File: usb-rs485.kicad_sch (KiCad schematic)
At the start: 8 parts

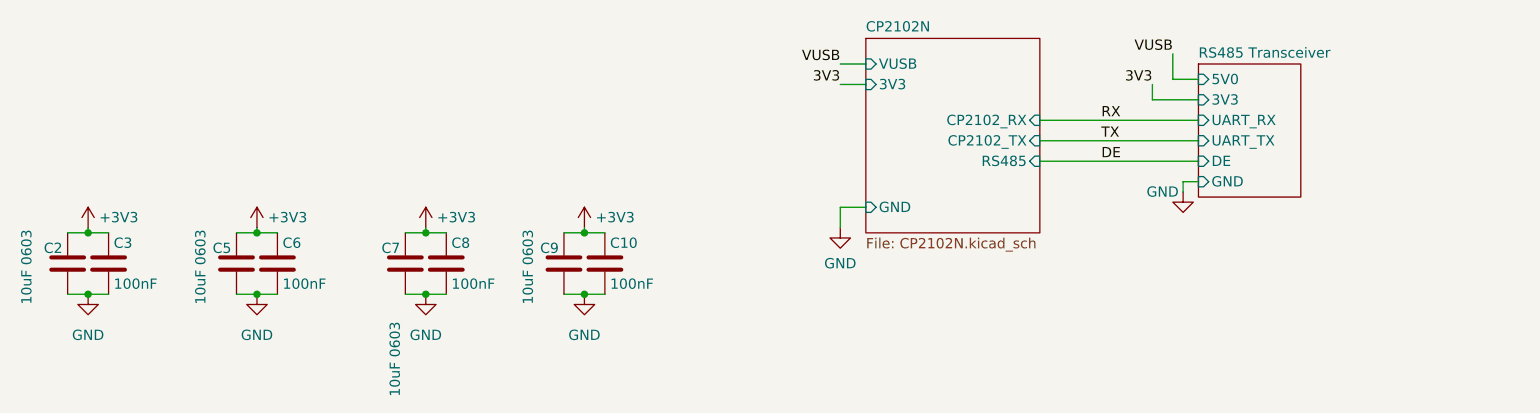
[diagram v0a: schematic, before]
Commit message: routing
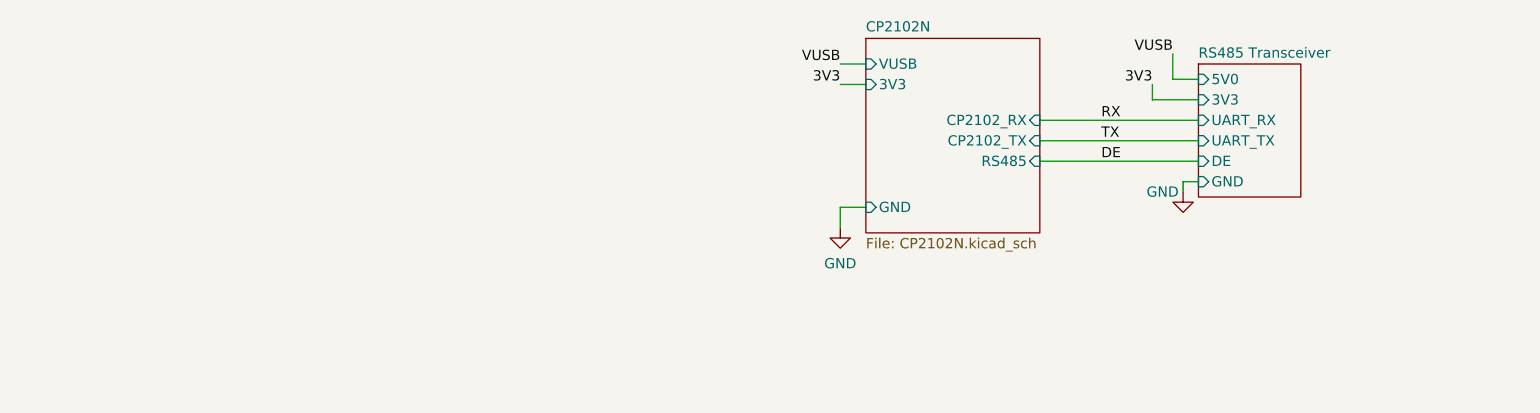
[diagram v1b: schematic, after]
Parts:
- removed C10, C3, C6, C8: 100nF, robot-cortex:C_0402_1005Metric, symbol usb-rs485:Capacitor
- removed C2, C5, C7, C9: 10uF 0603, robot-cortex:C_0603_1608Metric, symbol usb-rs485:Capacitor

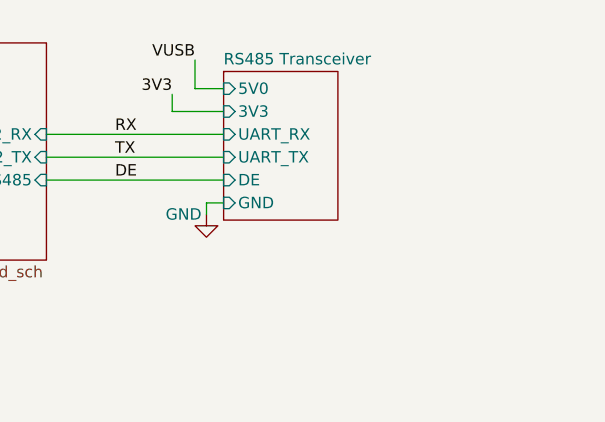
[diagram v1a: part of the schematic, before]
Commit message: routed, thru holes. ready to order i think
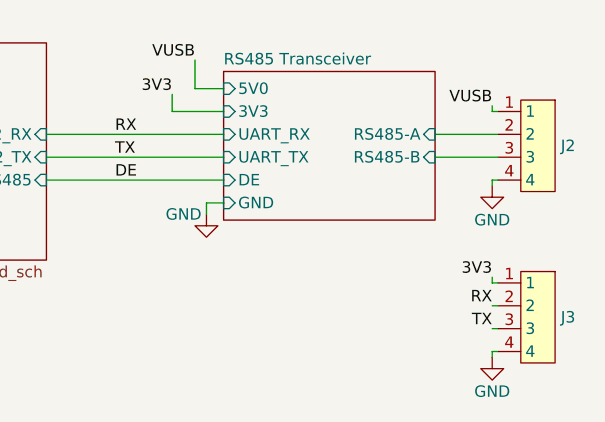
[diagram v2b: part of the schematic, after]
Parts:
- added J2, J3: ~, robot-cortex:ThruHoleBreadboardX4, symbol usb-rs485:ThruHoleX4
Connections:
- net 3V3: now also J3.1
- net GND: now also J2.4, J3.4
- net RX: now also J3.2
- net TX: now also J3.3
- net VUSB: now also J2.1
- new net RS485 Transceiver/RS485-A: J2.2
- new net RS485 Transceiver/RS485-B: J2.3
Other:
- sheet RS485 Transceiver ports: added RS485-A, RS485-B; removed none
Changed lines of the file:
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@@
 (kicad_sch (version 20230121) (generator eeschema)
   (paper "A3")
+  (wire (pts (xy 328.93 173.99) (xy 328.93 174.625))
+    (stroke (width 0) (type default))
+  )
+  (wire (pts (xy 328.93 154.94) (xy 328.93 155.575))
+    (stroke (width 0) (type default))
+  )
   (wire (pts (xy 295.91 144.78) (xy 299.085 144.78))
     (stroke (width 0) (type default))
   )
+  (wire (pts (xy 328.93 166.37) (xy 329.565 166.37))
+    (stroke (width 0) (type default))
+  )
+  (wire (pts (xy 328.93 173.99) (xy 329.565 173.99))
+    (stroke (width 0) (type default))
+  )
+  (wire (pts (xy 328.93 165.735) (xy 328.93 166.37))
+    (stroke (width 0) (type default))
+  )
   (wire (pts (xy 279.4 152.4) (xy 299.085 152.4))
     (stroke (width 0) (type default))
@@
     (stroke (width 0) (type default))
   )
+  (wire (pts (xy 322.58 149.86) (xy 329.565 149.86))
+    (stroke (width 0) (type default))
+  )
+  (wire (pts (xy 328.93 147.32) (xy 329.565 147.32))
+    (stroke (width 0) (type default))
+  )
   (wire (pts (xy 295.91 144.78) (xy 295.91 141.605))
     (stroke (width 0) (type default))
@@
     (stroke (width 0) (type default))
   )
+  (wire (pts (xy 322.58 152.4) (xy 329.565 152.4))
+    (stroke (width 0) (type default))
+  )
   (wire (pts (xy 279.4 149.86) (xy 299.085 149.86))
     (stroke (width 0) (type default))
   )
+  (wire (pts (xy 328.93 168.91) (xy 329.565 168.91))
+    (stroke (width 0) (type default))
+  )
+  (wire (pts (xy 328.93 171.45) (xy 329.565 171.45))
+    (stroke (width 0) (type default))
+  )
   (wire (pts (xy 297.18 157.48) (xy 297.18 158.75))
     (stroke (width 0) (type default))
@@
     (stroke (width 0) (type default))
   )
+  (wire (pts (xy 328.93 146.685) (xy 328.93 147.32))
+    (stroke (width 0) (type default))
+  )
+  (wire (pts (xy 328.93 154.94) (xy 329.565 154.94))
+    (stroke (width 0) (type default))
+  )
   (label "VUSB" (at 254.635 142.875 180) (fields_autoplaced)
+    (effects (font (size 1.27 1.27)) (justify right bottom))
+  )
+  (label "TX" (at 328.93 171.45 180) (fields_autoplaced)
     (effects (font (size 1.27 1.27)) (justify right bottom))
   )
@@
     (effects (font (size 1.27 1.27)) (justify right bottom))
   )
+  (label "RX" (at 328.93 168.91 180) (fields_autoplaced)
+    (effects (font (size 1.27 1.27)) (justify right bottom))
+  )
   (label "3V3" (at 293.37 145.415 180) (fields_autoplaced)
     (effects (font (size 1.27 1.27)) (justify right bottom))
@@
   (label "RX" (at 287.02 149.86 0) (fields_autoplaced)
     (effects (font (size 1.27 1.27)) (justify left bottom))
+  )
+  (label "VUSB" (at 328.93 146.685 180) (fields_autoplaced)
+    (effects (font (size 1.27 1.27)) (justify right bottom))
+  )
+  (label "3V3" (at 328.93 165.735 180) (fields_autoplaced)
+    (effects (font (size 1.27 1.27)) (justify right bottom))
   )
   (symbol (lib_id "power:GND") (at 297.18 158.75 0) (unit 1)
@@
     )
   )
-  (sheet (at 299.085 142.875) (size 12.7 16.51)
+  (symbol (lib_id "power:GND") (at 328.93 155.575 0) (unit 1)
+    (in_bom yes) (on_board yes) (dnp no)
+    (property "Reference" "#PWR011" (at 328.93 161.925 0)
+      (effects (font (size 1.27 1.27)) hide)
+    )
+    (property "Value" "GND" (at 328.93 159.385 0)
+      (effects (font (size 1.27 1.27)))
+    )
+    (property "Footprint" "" (at 328.93 155.575 0)
+      (effects (font (size 1.27 1.27)) hide)
+    )
+    (property "Datasheet" "" (at 328.93 155.575 0)
+      (effects (font (size 1.27 1.27)) hide)
+    )
+    (pin "1")
+    (instances
+      (project "usb-rs485"
+        (path "/19e4cb9f-d0a4-4ce0-8aa4-5fe95563dc37"
+          (reference "#PWR011") (unit 1)
+        )
+      )
+    )
+  )
+  (symbol (lib_id "usb-rs485:ThruHoleX4") (at 332.105 170.18 0) (mirror y) (unit 1)
+    (in_bom no) (on_board yes) (dnp no) (fields_autoplaced)
+    (property "Reference" "J3" (at 336.55 170.18 0)
+      (effects (font (size 1.27 1.27)) (justify right))
+    )
+    (property "Value" "~" (at 330.835 168.91 0)
+      (effects (font (size 1.27 1.27)))
+    )
+    (property "Footprint" "robot-cortex:ThruHoleBreadboardX4" (at 330.835 168.91 0)
+      (effects (font (size 1.27 1.27)) hide)
+    )
+    (property "Datasheet" "" (at 330.835 168.91 0)
+      (effects (font (size 1.27 1.27)) hide)
+    )
+    (pin "3")
+    (pin "4")
+    (pin "2")
+    (pin "1")
+    (instances
+      (project "usb-rs485"
+        (path "/19e4cb9f-d0a4-4ce0-8aa4-5fe95563dc37"
+          (reference "J3") (unit 1)
+        )
+      )
+    )
+  )
+  (symbol (lib_id "usb-rs485:ThruHoleX4") (at 332.105 151.13 0) (mirror y) (unit 1)
+    (in_bom no) (on_board yes) (dnp no) (fields_autoplaced)
+    (property "Reference" "J2" (at 336.55 151.13 0)
+      (effects (font (size 1.27 1.27)) (justify right))
+    )
+    (property "Value" "~" (at 330.835 149.86 0)
+      (effects (font (size 1.27 1.27)))
+    )
+    (property "Footprint" "robot-cortex:ThruHoleBreadboardX4" (at 330.835 149.86 0)
+      (effects (font (size 1.27 1.27)) hide)
+    )
+    (property "Datasheet" "" (at 330.835 149.86 0)
+      (effects (font (size 1.27 1.27)) hide)
+    )
+    (pin "3")
+    (pin "4")
+    (pin "2")
+    (pin "1")
+    (instances
+      (project "usb-rs485"
+        (path "/19e4cb9f-d0a4-4ce0-8aa4-5fe95563dc37"
+          (reference "J2") (unit 1)
+        )
+      )
+    )
+  )
+  (symbol (lib_id "power:GND") (at 328.93 174.625 0) (unit 1)
+    (in_bom yes) (on_board yes) (dnp no)
+    (property "Reference" "#PWR012" (at 328.93 180.975 0)
+      (effects (font (size 1.27 1.27)) hide)
+    )
+    (property "Value" "GND" (at 328.93 178.435 0)
+      (effects (font (size 1.27 1.27)))
+    )
+    (property "Footprint" "" (at 328.93 174.625 0)
+      (effects (font (size 1.27 1.27)) hide)
+    )
+    (property "Datasheet" "" (at 328.93 174.625 0)
+      (effects (font (size 1.27 1.27)) hide)
+    )
+    (pin "1")
+    (instances
+      (project "usb-rs485"
+        (path "/19e4cb9f-d0a4-4ce0-8aa4-5fe95563dc37"
+          (reference "#PWR012") (unit 1)
+        )
+      )
+    )
+  )
+  (sheet (at 299.085 142.875) (size 23.495 16.51)
     (stroke (width 0.1524) (type solid))
     (fill (color 0 0 0 0.0000))
@@
       (effects (font (size 1.27 1.27)) (justify left))
     )
-    (instances
+    (pin "RS485-B" input (at 322.58 152.4 0)
+      (effects (font (size 1.27 1.27)) (justify right))
+    )
+    (pin "RS485-A" input (at 322.58 149.86 0)
+      (effects (font (size 1.27 1.27)) (justify right))
+    )
+    (instances

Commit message: rename library to be for this
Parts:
- J2, J3: footprint robot-cortex:ThruHoleBreadboardX4 -> usb-rs485:ThruHoleBreadboardX4
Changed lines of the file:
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@@
       (effects (font (size 1.27 1.27)))
     )
-    (property "Footprint" "robot-cortex:ThruHoleBreadboardX4" (at 330.835 168.91 0)
+    (property "Footprint" "usb-rs485:ThruHoleBreadboardX4" (at 330.835 168.91 0)
       (effects (font (size 1.27 1.27)) hide)
     )
@@
       (effects (font (size 1.27 1.27)))
     )
-    (property "Footprint" "robot-cortex:ThruHoleBreadboardX4" (at 330.835 149.86 0)
+    (property "Footprint" "usb-rs485:ThruHoleBreadboardX4" (at 330.835 149.86 0)
       (effects (font (size 1.27 1.27)) hide)
     )
